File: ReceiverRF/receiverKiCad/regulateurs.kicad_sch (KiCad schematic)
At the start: 13 parts, among them J1 Conn_01x02

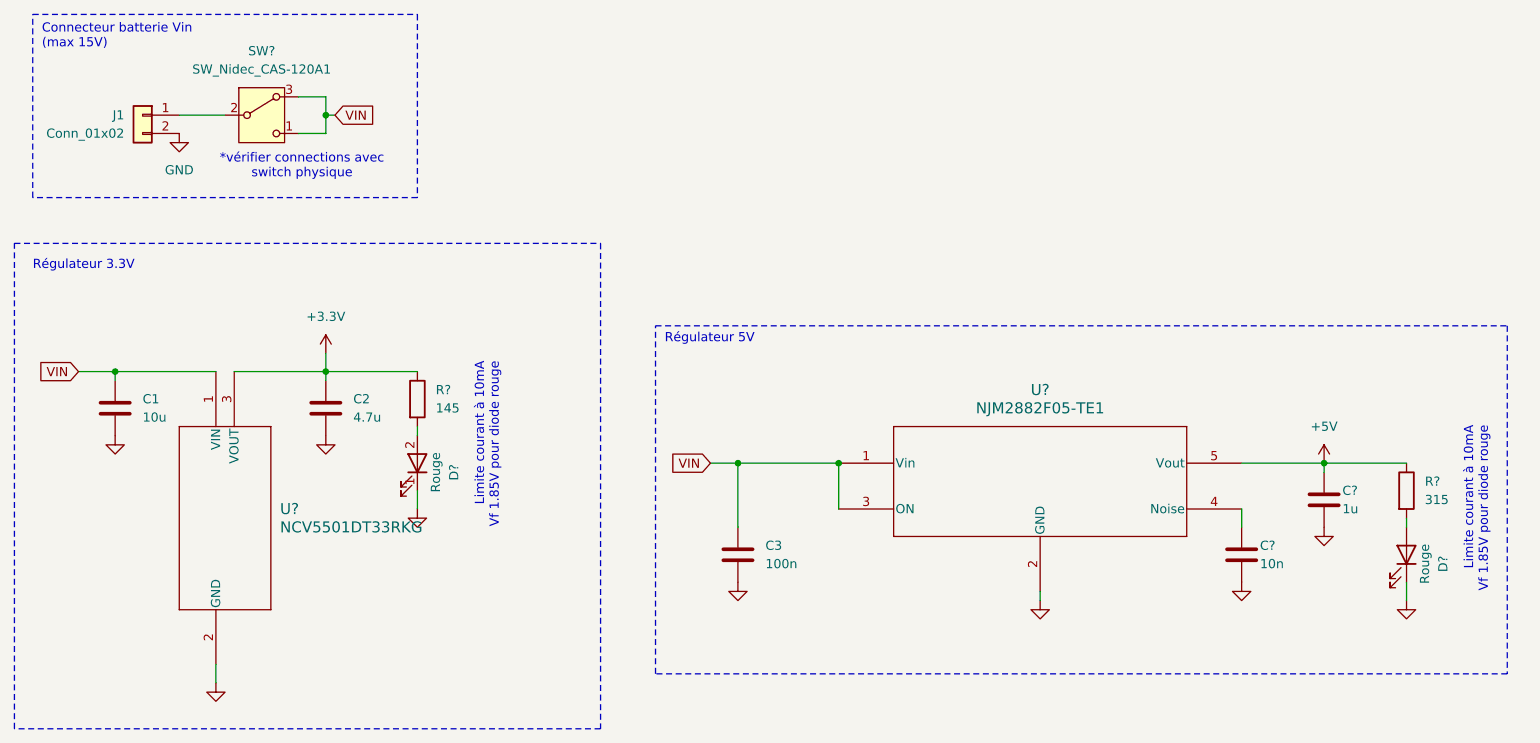
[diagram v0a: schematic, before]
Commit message: Identifiants des symboles
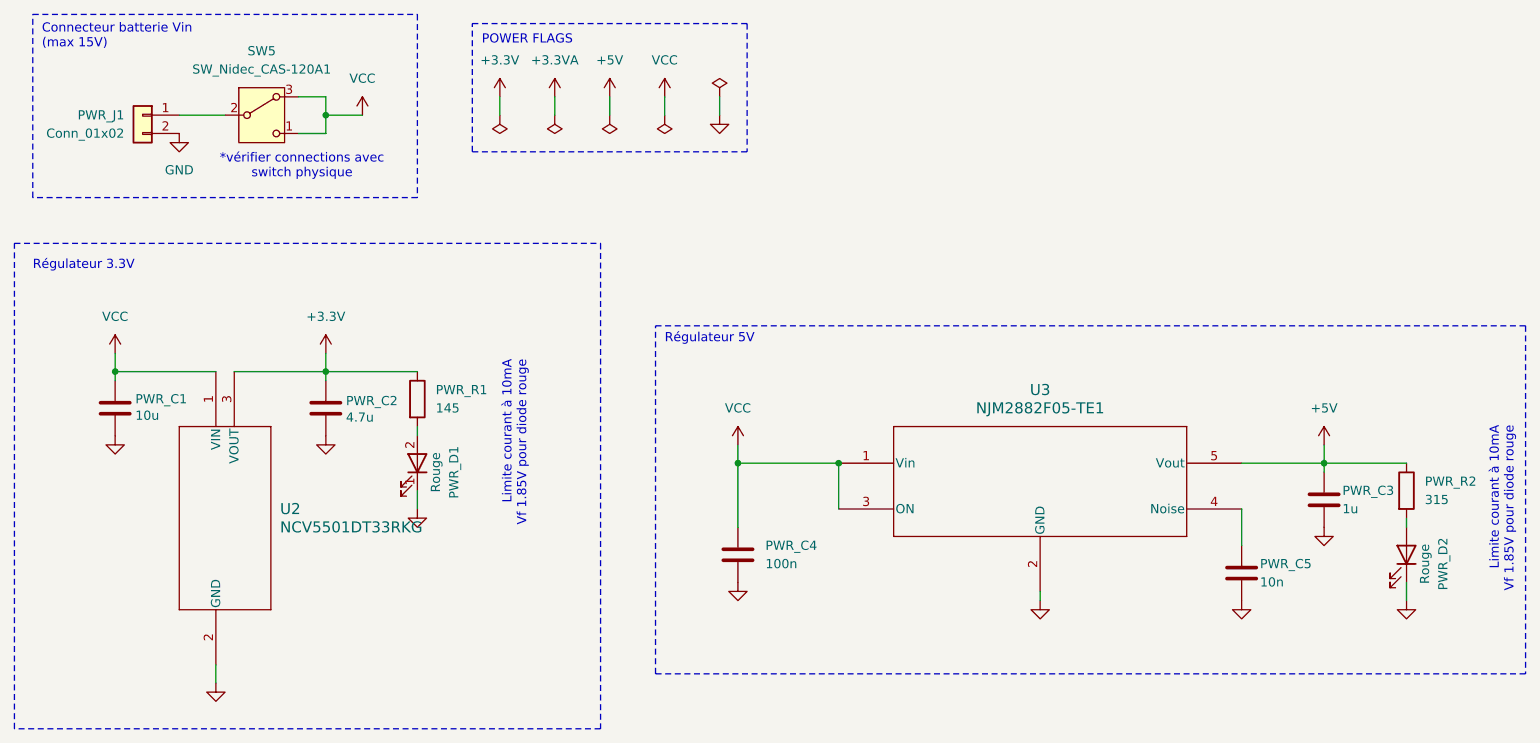
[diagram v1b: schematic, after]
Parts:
- gave numbers to parts that had none: 9
- renumbered C1 to PWR_C1, C2 to PWR_C2, C3 to PWR_C4, J1 to PWR_J1
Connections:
- net VIN renamed VCC
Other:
- note added: "POWER FLAGS"
- moved on the sheet: PWR_C5
